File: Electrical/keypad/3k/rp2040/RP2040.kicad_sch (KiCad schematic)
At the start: 73 parts, among them J1 Conn_01x04_Socket, P1 USB-TYPE-C-016, Q1 BSS138, SW1 TS-1187A-B-A-B, SW2 TS-1187A-B-A-B, SW3 BUTT1, SW4 BUTT2, SW5 BUTT3, U1 PRTR5V0U2X, U2 ME6208A44M3G, U3 RP2040, U4 ME6212C25M5G, U5 W25Q16JVSS, U6 ME6212C33M5G, U7 SLSS49E, U8 SLSS49E, U9 SLSS49E, Y1 12MHz

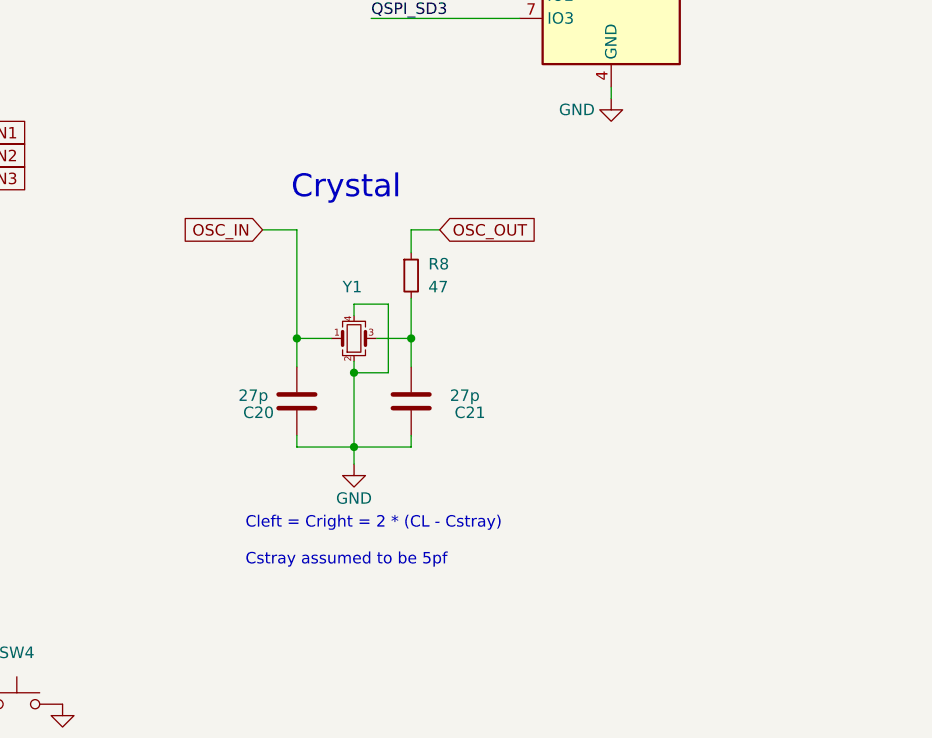
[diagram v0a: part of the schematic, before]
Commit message: saves latest progress
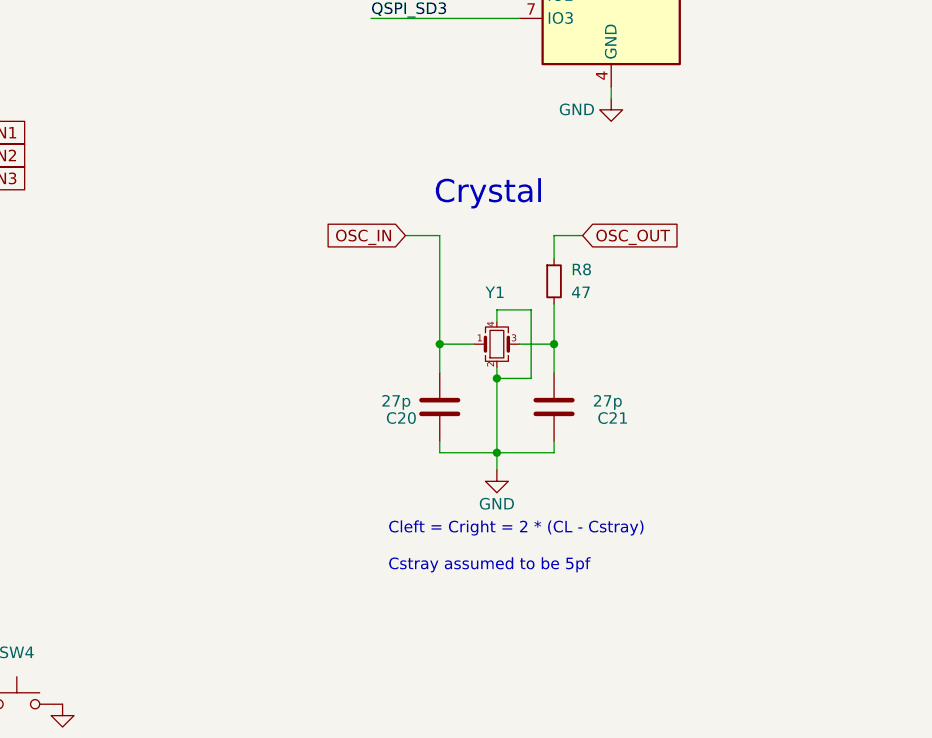
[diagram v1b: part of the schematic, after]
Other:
- moved on the sheet: C20, C21, R8, Y1
